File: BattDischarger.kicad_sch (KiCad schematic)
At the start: 33 parts, among them J1 Conn_01x02, J10 Conn_01x02, J8 Conn_01x03, J9 Conn_01x02, Q2 Q_NMOS_DGS, SW3 RA12131100, SW5 SW_SPDT, U3 OP179GRT, U4 OP179GRT, U8 OP179GRT

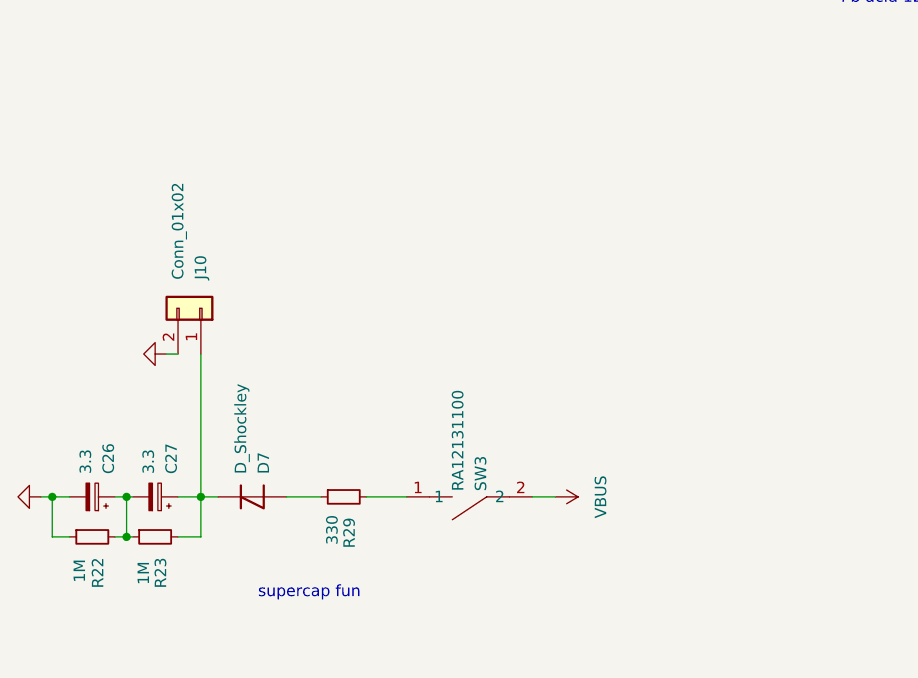
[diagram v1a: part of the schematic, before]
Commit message: j
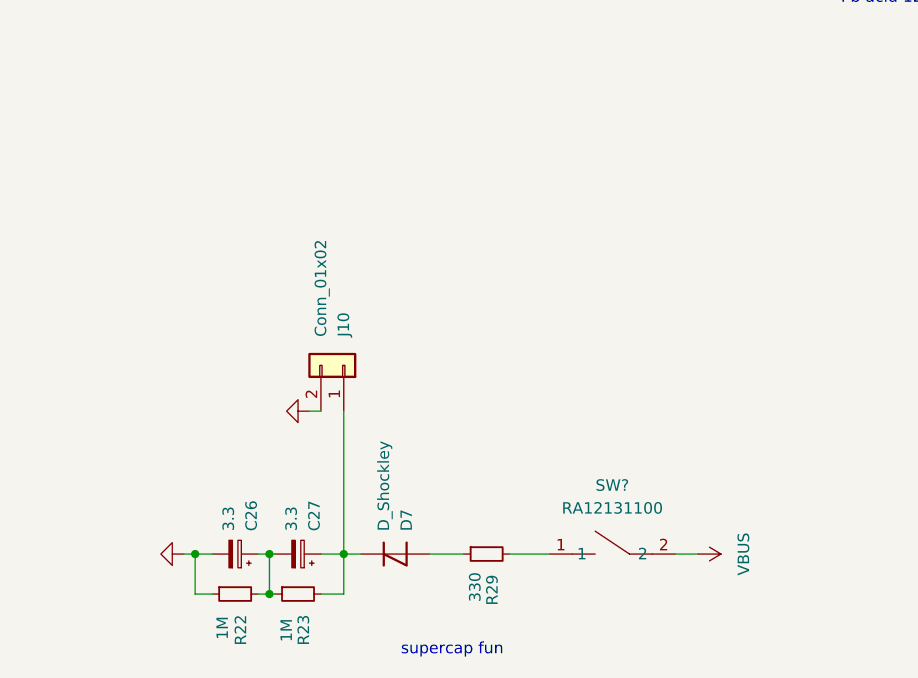
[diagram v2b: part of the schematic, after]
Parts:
- removed SW3: RA12131100, symbol My_custom_lib:RA12131100
- added SW?: RA12131100, Z_mycustom_footprint_lib:RA12131100, symbol My_custom_lib:RA12131100
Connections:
- net VBUS: now also SW?.2
- net at R29.2: now also SW?.1
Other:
- moved on the sheet: C26, C27, D7, J10, R22, R23, R29
